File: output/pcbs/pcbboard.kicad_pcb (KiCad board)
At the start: 2 copper layers, 151.2 x 121.7 mm, 49 parts

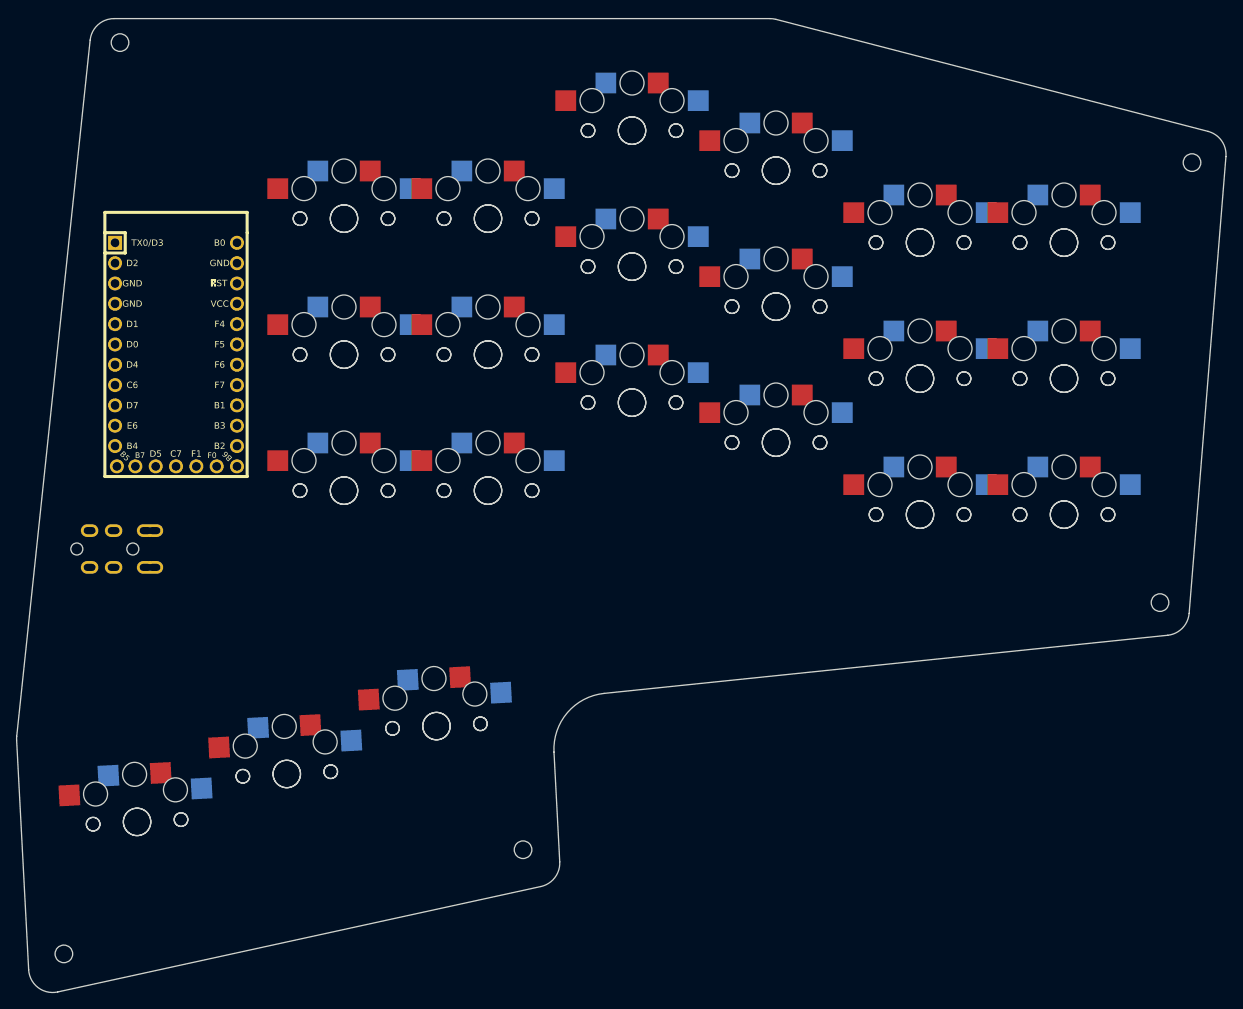
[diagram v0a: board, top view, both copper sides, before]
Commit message: PCB redesign
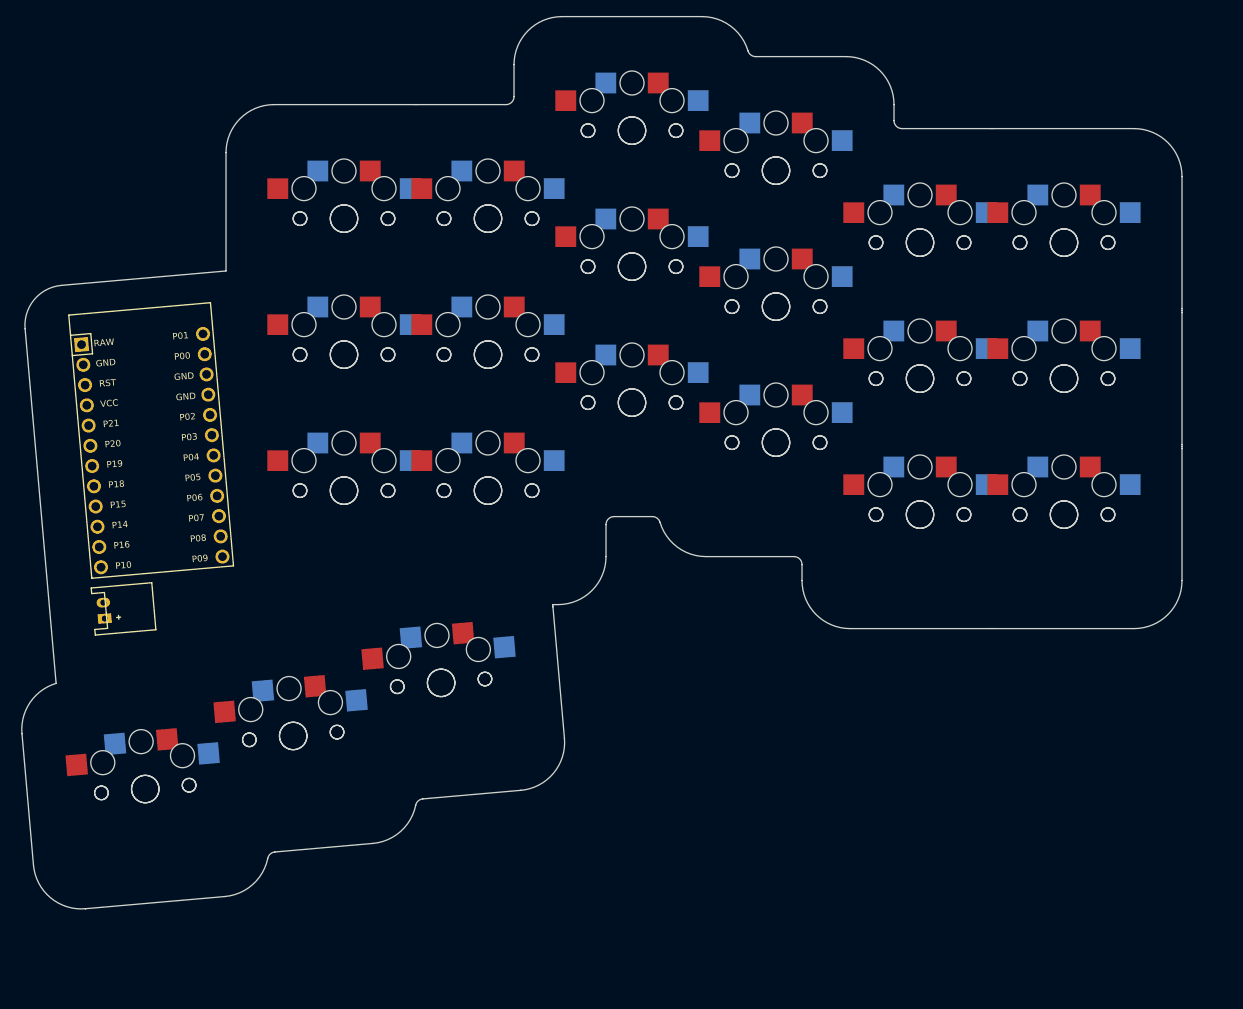
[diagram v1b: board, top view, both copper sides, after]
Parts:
- removed TRRS1: TRRS-PJ-320A-dual, TRRS-PJ-320A-dual
- removed _1, _2, _3, _4, _5: , MountingHole_2.2mm_M2
- added JST1: , JST_PH_S2B-PH-K_02x2.00mm_Angled, F.Cu at (-30.0, 15.0)
- MCU1: value Elite-C -> (none); footprint Elite-C -> ProMicro
- moved MCU1 12.4 mm to (-24.0, -5.00), turned to -85 degrees
- moved S21 5.43 mm to (12.1, 24.0), turned to 5 degrees
- moved S42 5.43 mm to (12.1, 24.0), turned to 5 degrees
- moved S20 4.82 mm to (-6.35, 30.7), turned to 5 degrees
- moved S41 4.82 mm to (-6.35, 30.7), turned to 5 degrees
- moved S19 4.23 mm to (-24.8, 37.3), turned to 5 degrees
- moved S40 4.23 mm to (-24.8, 37.3), turned to 5 degrees
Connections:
- net D3 renamed RAW
- MCU1 pad 10: matrix_pinky_bottom -> matrix_middle_bottom
- MCU1 pad 11: matrix_ring_bottom -> matrix_pointer_bottom
- MCU1 pad 12: matrix_middle_bottom -> matrix_inner_bottom
- MCU1 pad 13: matrix_middle_center -> matrix_outer_middle
- MCU1 pad 14: matrix_pointer_center -> matrix_ring_middle
- MCU1 pad 15: matrix_inner_center -> GND
- MCU1 pad 16: matrix_outer_top -> GND
- MCU1 pad 17: matrix_pinky_top -> matrix_middle_middle
- MCU1 pad 18: matrix_ring_top -> matrix_pointer_middle
- MCU1 pad 19: matrix_middle_top -> matrix_inner_middle
- MCU1 pad 2: D2 -> GND
- MCU1 pad 20: matrix_pointer_top -> matrix_outer_top
- MCU1 pad 21: VCC -> matrix_ring_top
- MCU1 pad 22: ST -> matrix_middle_top
- MCU1 pad 23: GND -> matrix_pointer_top
- MCU1 pad 3: GND -> RST
- MCU1 pad 4: GND -> VCC
- MCU1 pad 5: D1 -> thumb_left
- MCU1 pad 6: thumb_left -> thumb_middle
- MCU1 pad 7: thumb_middle -> thumb_right
- MCU1 pad 8: thumb_right -> matrix_outer_bottom
- MCU1 pad 9: matrix_outer_bottom -> matrix_ring_bottom
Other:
- board size 151.2 x 121.7 mm -> 145 x 111.5 mm
